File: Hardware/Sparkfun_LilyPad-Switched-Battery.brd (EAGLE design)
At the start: 31.6 x 30 mm, 11 parts

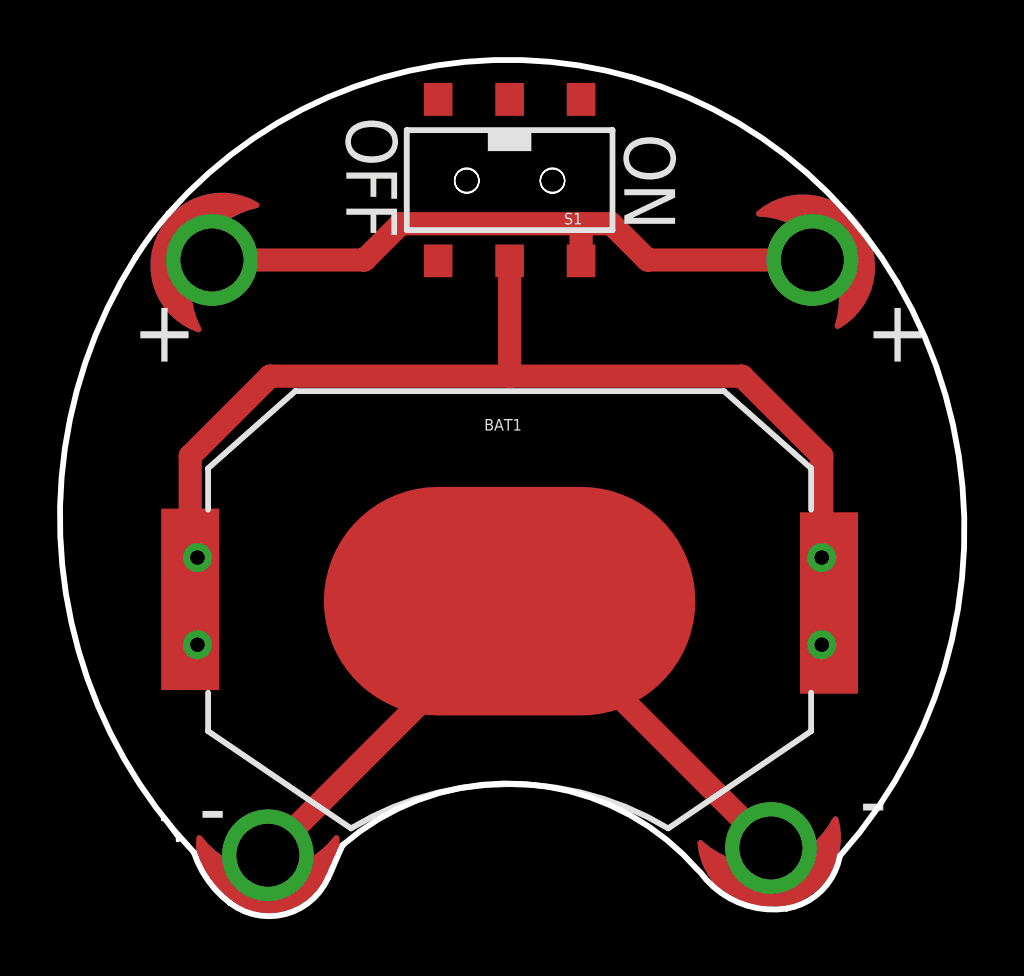
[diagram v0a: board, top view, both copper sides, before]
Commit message: Updated Brd files per Eng Design Review
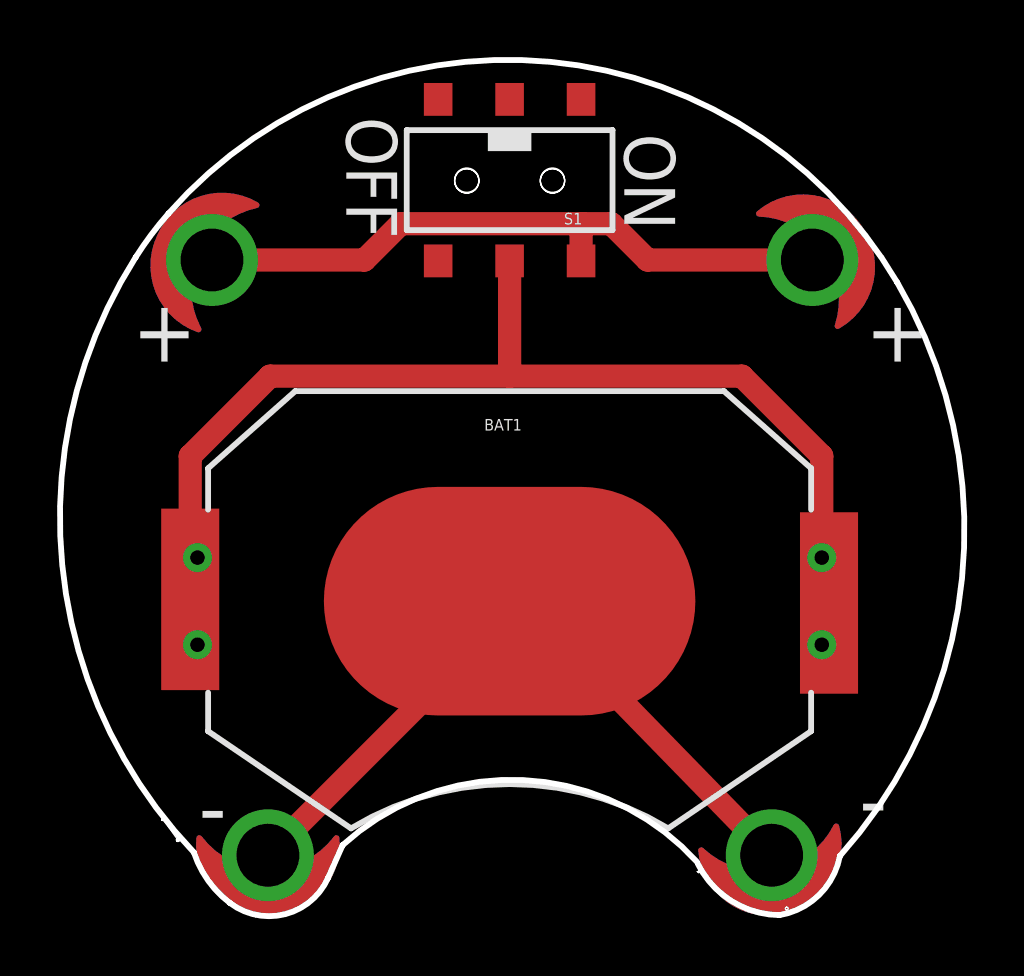
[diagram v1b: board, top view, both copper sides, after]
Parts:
- moved BATB-2 0.26 mm to (22.9, 2.03)
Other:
- outline, holes or cut-outs redrawn
- board text added: "Purple Silk"
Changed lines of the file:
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@@
 <setting verticaltext="up"/>
 </settings>
-<grid distance="0.05" unitdist="inch" unit="inch" style="lines" multiple="1" display="yes" altdistance="0.005" altunitdist="inch" altunit="inch"/>
+<grid distance="0.001" unitdist="inch" unit="inch" style="lines" multiple="1" display="yes" altdistance="0.005" altunitdist="inch" altunit="inch"/>
 <layers>
 <layer number="1" name="Top" color="4" fill="1" visible="yes" active="yes"/>
@@
 <wire x1="3.9676" y1="0.3961" x2="3.9064" y2="0.3151" width="0.008" layer="20" curve="180"/>
 <wire x1="7.4125" y1="1.224" x2="7.3195" y2="1.2652" width="0.008" layer="20" curve="180"/>
-<wire x1="20.3784" y1="1.4503" x2="23.4112" y2="0.1651" width="0.008" layer="20" curve="62.8"/>
+<wire x1="20.3022" y1="1.7297" x2="23.1572" y2="-0.0635" width="0.008" layer="20" curve="62.8"/>
 <wire x1="20.4197" y1="1.4799" x2="20.3371" y2="1.4207" width="0.008" layer="20" curve="180"/>
 <wire x1="7.9204" y1="2.367" x2="7.8276" y2="2.4082" width="0.008" layer="20" curve="180"/>
 <wire x1="7.3196" y1="1.2652" x2="7.4124" y2="1.224" width="0.008" layer="20" curve="180"/>
-<wire x1="20.32" y1="1.4986" x2="7.874" y2="2.3876" width="0.008" layer="20" curve="90"/>
+<wire x1="20.2692" y1="1.8034" x2="7.874" y2="2.3876" width="0.008" layer="20" curve="90"/>
 <wire x1="20.2816" y1="1.4653" x2="20.3584" y2="1.5319" width="0.008" layer="20" curve="180"/>
 <wire x1="7.8407" y1="2.426" x2="7.9073" y2="2.3492" width="0.008" layer="20" curve="180"/>
@@
 <wire x1="27.2358" y1="22.0468" x2="27.3234" y2="22.0984" width="0.008" layer="20" curve="180"/>
 <wire x1="1.7398" y1="24.5191" x2="1.8162" y2="24.4521" width="0.008" layer="20" curve="180"/>
-<wire x1="23.4112" y1="0.1651" x2="25.273" y2="2.0066" width="0.2032" layer="20" curve="69.88"/>
+<wire x1="23.1572" y1="-0.0635" x2="25.273" y2="2.0066" width="0.2032" layer="20" curve="69.88"/>
 <wire x1="25.323" y1="1.9974" x2="25.223" y2="2.0158" width="0.008" layer="20" curve="180"/>
 <wire x1="25.273" y1="2.0066" x2="27.2796" y2="22.0726" width="0.2032" layer="20" curve="72.18"/>
@@
 <wire x1="3.9676" y1="0.3961" x2="3.9064" y2="0.3151" width="0.008" layer="20" curve="180"/>
 <wire x1="7.4125" y1="1.224" x2="7.3195" y2="1.2652" width="0.008" layer="20" curve="180"/>
-<wire x1="20.3784" y1="1.4503" x2="23.4112" y2="0.1651" width="0.2032" layer="20" curve="62.8"/>
+<wire x1="20.3022" y1="1.7297" x2="23.1572" y2="-0.0635" width="0.2032" layer="20" curve="62.8"/>
 <wire x1="20.4197" y1="1.4799" x2="20.3371" y2="1.4207" width="0.008" layer="20" curve="180"/>
 <wire x1="23.4186" y1="0.1148" x2="23.4038" y2="0.2154" width="0.008" layer="20" curve="180"/>
@@
 <wire x1="7.9204" y1="2.367" x2="7.8276" y2="2.4082" width="0.008" layer="20" curve="180"/>
 <wire x1="7.3196" y1="1.2652" x2="7.4124" y2="1.224" width="0.008" layer="20" curve="180"/>
-<wire x1="20.32" y1="1.4986" x2="7.874" y2="2.3876" width="0.2032" layer="20" curve="90"/>
+<wire x1="20.2692" y1="1.8034" x2="7.874" y2="2.3876" width="0.2032" layer="20" curve="90"/>
 <wire x1="20.2816" y1="1.4653" x2="20.3584" y2="1.5319" width="0.008" layer="20" curve="180"/>
 <wire x1="7.8407" y1="2.426" x2="7.9073" y2="2.3492" width="0.008" layer="20" curve="180"/>
@@
 <wire x1="27.2358" y1="22.0468" x2="27.3234" y2="22.0984" width="0.008" layer="20" curve="180"/>
 <wire x1="1.7398" y1="24.5191" x2="1.8162" y2="24.4521" width="0.008" layer="20" curve="180"/>
-<wire x1="23.4112" y1="0.1651" x2="25.273" y2="2.0066" width="0.008" layer="20" curve="69.88"/>
+<wire x1="23.1572" y1="-0.0635" x2="25.273" y2="2.0066" width="0.008" layer="20" curve="69.88"/>
 <wire x1="23.4026" y1="0.2152" x2="23.4198" y2="0.115" width="0.008" layer="20" curve="180"/>
 <wire x1="25.323" y1="1.9974" x2="25.223" y2="2.0158" width="0.008" layer="20" curve="180"/>
@@
 <text x="3.81" y="4.826" size="2.1844" layer="21" font="vector" ratio="15" rot="R180">-</text>
 <text x="26.924" y="5.08" size="2.1844" layer="21" font="vector" ratio="15" rot="R180">-</text>
-<text x="24.384" y="5.08" size="1.016" layer="22" font="vector" ratio="15" rot="MR180">-</text>
+<text x="24.384" y="5.08" size="2.1844" layer="22" font="vector" ratio="15" rot="MR180">-</text>
 <text x="1.27" y="4.826" size="2.1844" layer="22" font="vector" ratio="15" rot="MR180">-</text>
 <rectangle x1="12.954" y1="26.67" x2="14.478" y2="27.432" layer="21"/>
@@
 <dimension x1="3.302" y1="22.86" x2="24.3078" y2="22.86" x3="13.8049" y3="32.766" textsize="1.778" textratio="15" layer="47" unit="inch"/>
 <dimension x1="24.3078" y1="22.86" x2="22.86" y2="2.286" x3="34.43429375" y3="11.809453125" textsize="1.778" textratio="15" layer="47" unit="inch"/>
+<text x="33.02" y="30.48" size="1.778" layer="47" font="vector" ratio="15">Purple Silk</text>
+<dimension x1="5.2578" y1="2.032" x2="22.8854" y2="2.032" x3="14.0716" y3="-1.27" textsize="1.778" textratio="15" layer="47" unit="inch"/>
 </plain>
 <attributes>
@@
 </element>
 <element name="BATB-" library="LilyPad-Wearables" package="PETAL-SMALL-2SIDE" value="SEWTAP6" x="5.2578" y="2.032"/>
-<element name="BATB-2" library="LilyPad-Wearables" package="PETAL-SMALL-2SIDE" value="SEWTAP6" x="22.86" y="2.286" rot="R10"/>
+<element name="BATB-2" library="LilyPad-Wearables" package="PETAL-SMALL-2SIDE" value="SEWTAP6" x="22.8854" y="2.032" rot="R10"/>
 <element name="BATT+" library="LilyPad-Wearables" package="PETAL-SMALL-2SIDE" value="SEWTAP6" x="3.302" y="22.86" rot="R245"/>
 <element name="BATT+2" library="LilyPad-Wearables" package="PETAL-SMALL-2SIDE" value="SEWTAP6" x="24.3078" y="22.86" rot="R125"/>
@@
 <wire x1="13.716" y1="10.922" x2="13.716" y2="10.4902" width="0.8128" layer="1"/>
 <wire x1="13.716" y1="10.922" x2="14.224" y2="10.922" width="0.8128" layer="1"/>
-<wire x1="14.224" y1="10.922" x2="22.86" y2="2.286" width="0.8128" layer="1"/>
+<wire x1="14.224" y1="10.922" x2="22.8854" y2="2.032" width="0.8128" layer="1"/>
 <wire x1="13.716" y1="10.4902" x2="5.2578" y2="2.032" width="0.8128" layer="1"/>
 </signal>
